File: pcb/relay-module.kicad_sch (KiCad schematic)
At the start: 12 parts

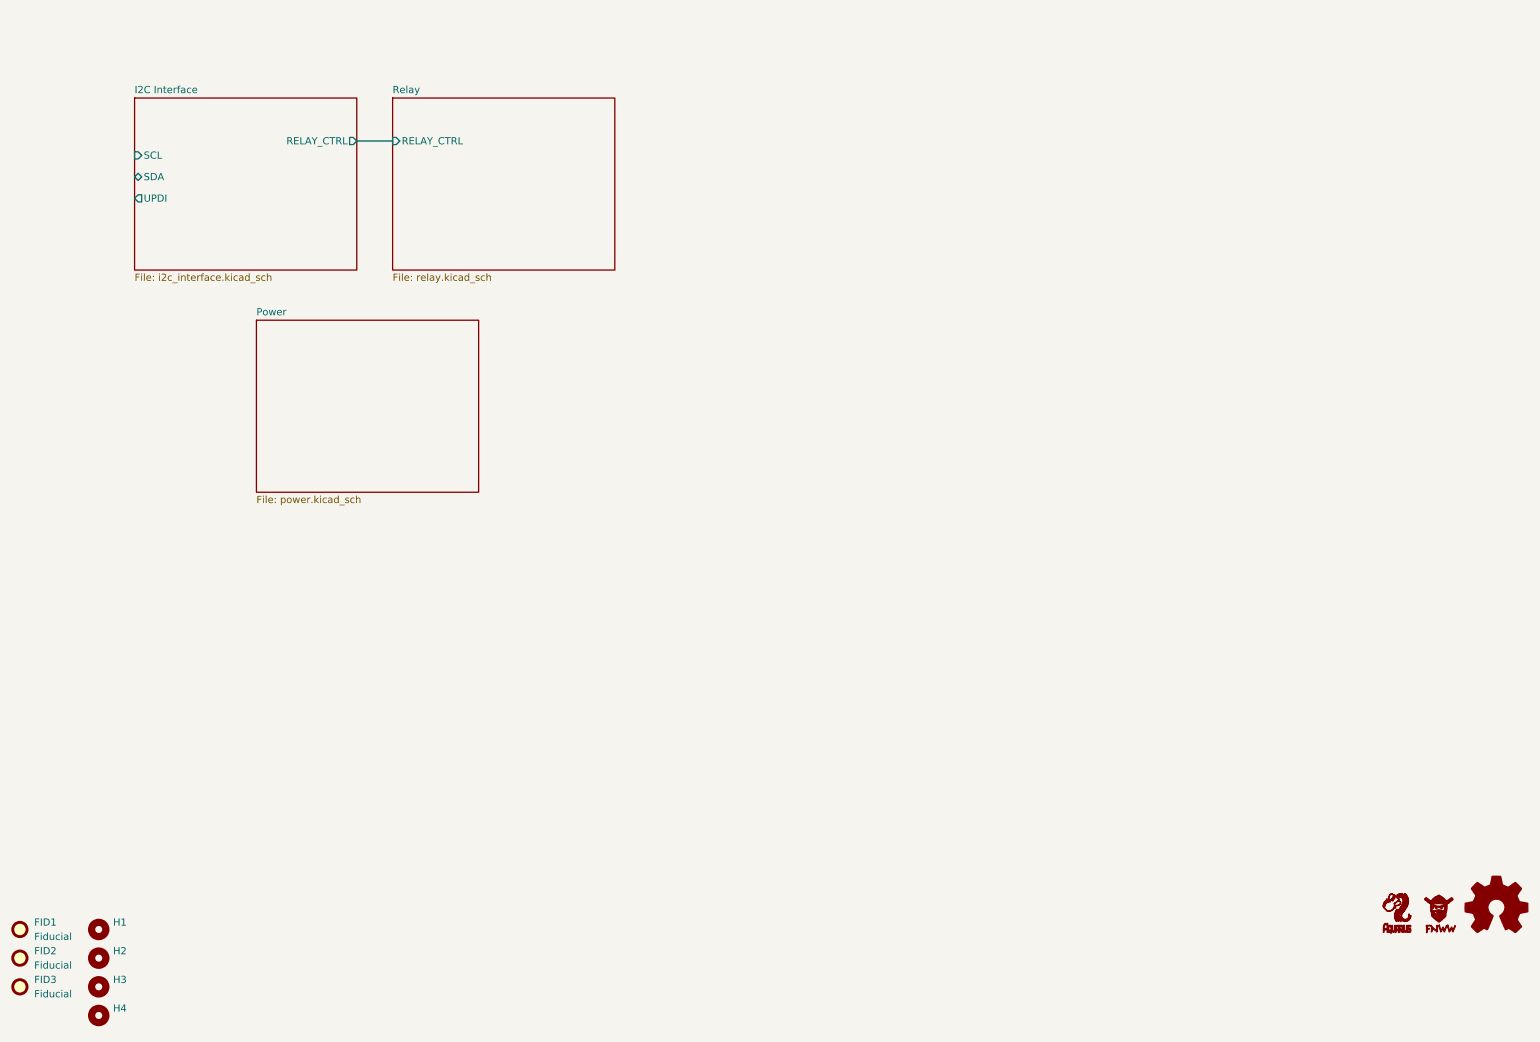
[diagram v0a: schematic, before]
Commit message: initial checkin
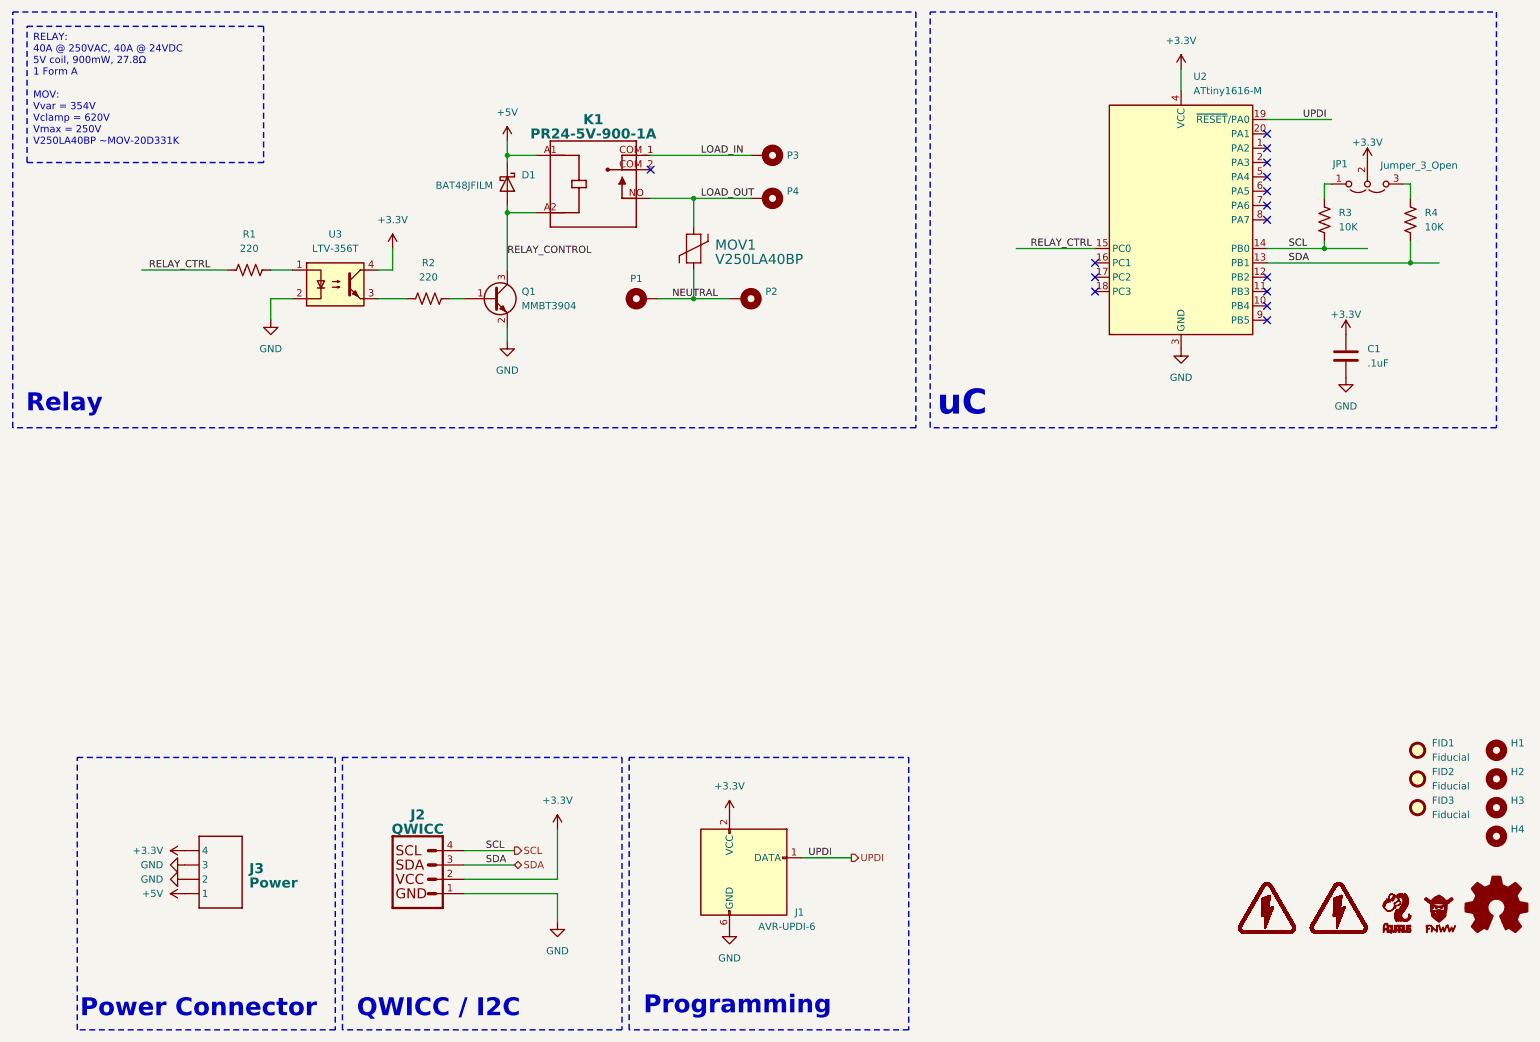
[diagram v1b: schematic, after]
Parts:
- added C1: .1uF, Capacitor_SMD:C_0603_1608Metric, symbol Device:C
- added D1: BAT48JFILM, Diode_SMD:D_SOD-323, symbol Diode:BAT48JFILM
- added J1: AVR-UPDI-6, Connector_PinHeader_2.54mm:PinHeader_2x03_P2.54mm_Vertical, symbol Connector:AVR-UPDI-6
- added J2: QWICC, Connector_JST:JST_SH_SM04B-SRSS-TB_1x04-1MP_P1.00mm_Horizontal, symbol CRGM Connector:QWIIC
- added J3: Power, Connector_JST:JST_SH_SM04B-SRSS-TB_1x04-1MP_P1.00mm_Horizontal, symbol CRGM Connector:JST-SH-4
- added JP1: Jumper_3_Open, Jumper:SolderJumper-3_P1.3mm_Open_RoundedPad1.0x1.5mm_NumberLabels, symbol Jumper:Jumper_3_Open
- added K1: PR24-5V-900-1A, CRG Makes:RELAY_PR24-5V-900-1A, symbol CRG Makes:PR24-5V-900-1A
- added MOV1: V250LA40BP, CRG Makes:V250LA40BP, symbol CRG Makes:MOV20D331K
- added P1, P2, P3, P4: MountingHole_Pad, MountingHole:MountingHole_3.2mm_M3_ISO14580_Pad, symbol Mechanical:MountingHole_Pad
- added Q1: MMBT3904, Package_TO_SOT_SMD:SOT-23, symbol Transistor_BJT:MMBT3904
- added R1, R2: 220, Resistor_SMD:R_0603_1608Metric, symbol Device:R_US
- added R3, R4: 10K, Resistor_SMD:R_0603_1608Metric, symbol Device:R_US
- added S1, S2: ~, CRGM Symbols:HIGH-VOLTAGE-5MM, symbol CRGM Symbols:High Voltage
- added U2: ATtiny1616-M, Package_DFN_QFN:VQFN-20-1EP_3x3mm_P0.4mm_EP1.7x1.7mm, symbol MCU_Microchip_ATtiny:ATtiny1616-M
- added U3: LTV-356T, Package_SO:SO-4_4.4x3.6mm_P2.54mm, symbol Isolator:LTV-356T
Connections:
- new net: R1.2, U3.1
- new net: R2.1, U3.3
- new net: JP1.1 (A), R3.2
- new net: JP1.3 (B), R4.2
- new net: Q1.1 (B), R2.2
- new net +3.3V: C1.1, J1.2 (VCC), J2.2, J3.4, JP1.2 (C), U2.4 (VCC), U3.4
- new net +5V: D1.1 (K), J3.1, K1.A1 (COIL1)
- new net GND: C1.2, J1.6 (GND), J2.1, J3.2, J3.3, Q1.2 (E), U2.21 (GND), U2.3 (GND), U3.2
- new net LOAD_IN: K1.COM_1 (COM1), P3.1
- new net LOAD_OUT: K1.NO, MOV1.P$1, P4.1
- new net NEUTRAL: MOV1.P$2, P1.1, P2.1
- new net RELAY_CONTROL: D1.2 (A), K1.A2 (COIL2), Q1.3 (C)
- new net RELAY_CTRL: R1.1, U2.15 (PC0)
- new net SCL: J2.4, R3.1, U2.14 (PB0)
- new net SDA: J2.3, R4.1, U2.13 (PB1)
- new net UPDI: J1.1 (DATA), U2.19 (~{RESET}/PA0)
- no-connect marks 0 -> 15
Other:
- removed sheet I2C Interface
- removed sheet Power
- removed sheet Relay
- note added: "Power Connector"
- note added: "Programming"
- note added: "QWICC / I2C"
- note added: "Relay"
- note added: "uC"
- moved on the sheet: FID1, FID2, FID3, H1, H2, H3, H4
